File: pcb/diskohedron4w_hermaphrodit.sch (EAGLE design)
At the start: 20 parts, among them X1 87758-1216, X2 87758-1216

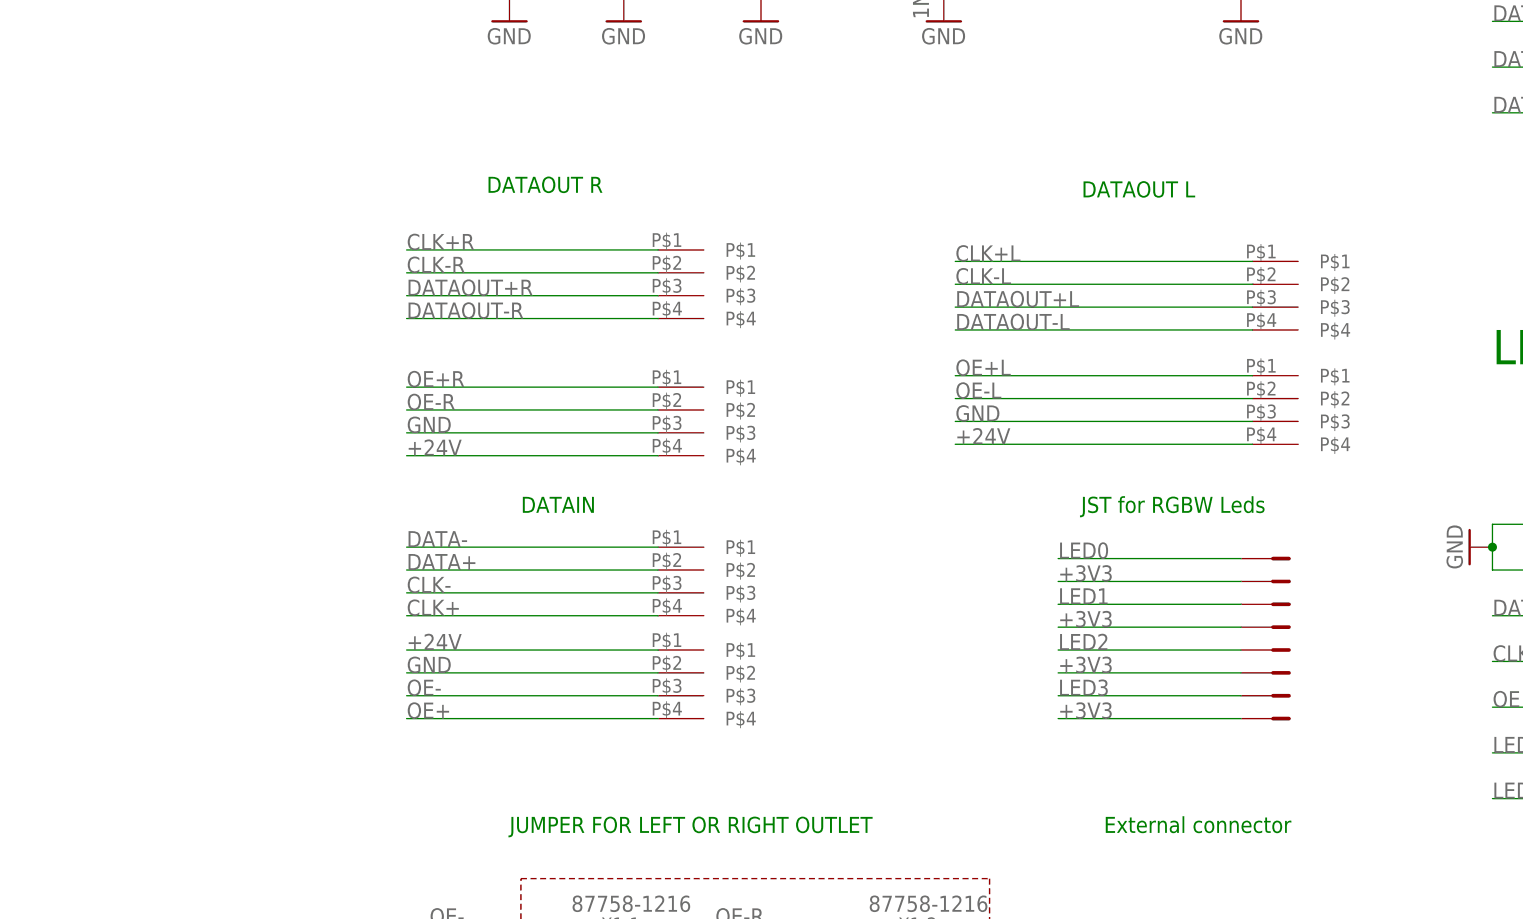
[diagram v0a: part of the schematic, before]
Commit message: updated pcb
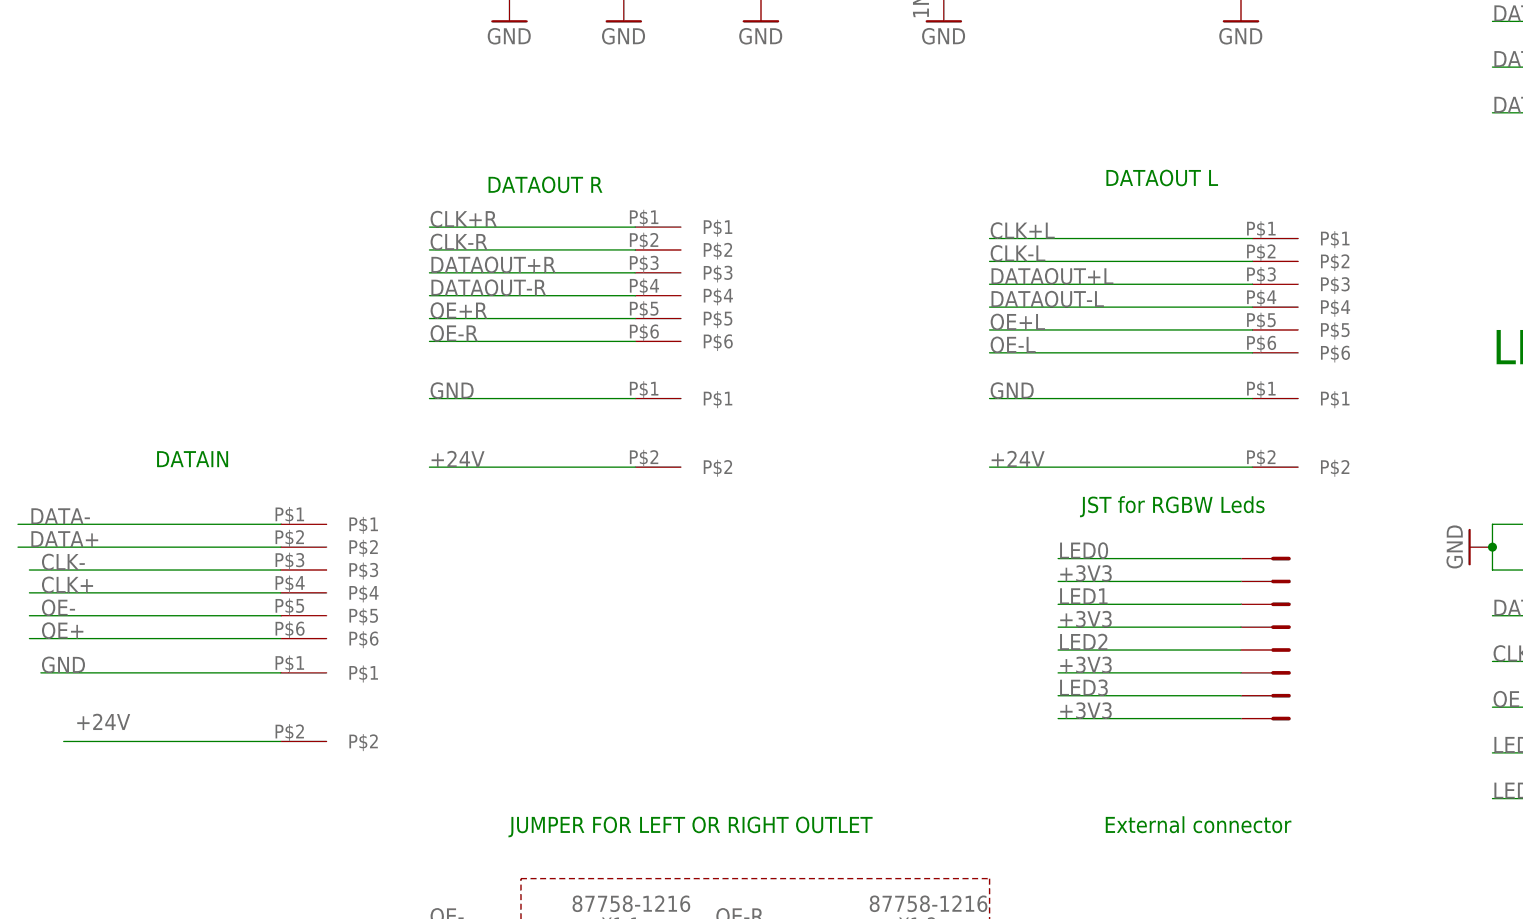
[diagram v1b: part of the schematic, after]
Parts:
- removed IN1, IN2, OUTR1, OUTR2, U$10, U$9: HERMAPHRODIT4PIN, diskohedron:HERMAPHRODIT4PIN
- added U$11, U$5, U$8: HERMAPHRODITMINI6PIN, diskohedron:HERMAPHRODITMINI6PIN
- added U$12, U$6, U$7: HERMAPHRODIT2PIN, diskohedron:HERMAPHRODIT2PIN
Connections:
- net +24V: now also U$12.P$2, U$6.P$2, U$7.P$2; no longer IN2.P$1, OUTR2.P$4, U$10.P$4
- net CLK+: now also U$8.P$4; no longer IN1.P$4
- net CLK+L: now also U$11.P$1; no longer U$9.P$1
- net CLK+R: now also U$5.P$1; no longer OUTR1.P$1
- net CLK-: now also U$8.P$3; no longer IN1.P$3
- net CLK-L: now also U$11.P$2; no longer U$9.P$2
- net CLK-R: now also U$5.P$2; no longer OUTR1.P$2
- net DATA+: now also U$8.P$2; no longer IN1.P$2
- net DATA-: now also U$8.P$1; no longer IN1.P$1
- net DATAOUT+L: now also U$11.P$3; no longer U$9.P$3
- net DATAOUT+R: now also U$5.P$3; no longer OUTR1.P$3
- net DATAOUT-L: now also U$11.P$4; no longer U$9.P$4
- net DATAOUT-R: now also U$5.P$4; no longer OUTR1.P$4
- net GND: now also U$12.P$1, U$6.P$1, U$7.P$1; no longer IN2.P$2, OUTR2.P$3, U$10.P$3
- net OE+: now also U$8.P$6; no longer IN2.P$4
- net OE+L: now also U$11.P$5; no longer U$10.P$1
- net OE+R: now also U$5.P$5; no longer OUTR2.P$1
- net OE-: no longer IN2.P$3
- net OE-L: now also U$11.P$6; no longer U$10.P$2
- net OE-R: now also U$5.P$6; no longer OUTR2.P$2
